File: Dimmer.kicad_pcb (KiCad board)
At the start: 2 copper layers, 129 x 68 mm, 62 parts, among them J1 220to12, J10 Detect_nullA, J11 220v_OUT, J12 Load_cntrlA, J13 ADC, J14 Conn_01x01, J15 Conn_01x01, J16 Conn_01x01, J17 Conn_01x01, J18 Conn_01x01, J19 Conn_01x01, J2 Prog, J22 SPI, J3 UART0, J4 Mode, J5 Load_cntrl, J6 Detect_null, J7 I2C, J8 ADC, J9 220v_IN, Q1 IRFP460APBF, Q2 IRFP460APBF, Q3 BC807, SW1 SW_Push, SW2 SW_Push, U2 ESP32-WROOM-32D, U3 L78L33_SO8, U4 TLP185, k1 Key, k2 Key, k3 Key, k4 Key, k5 Key, k6 Key, k7 Key

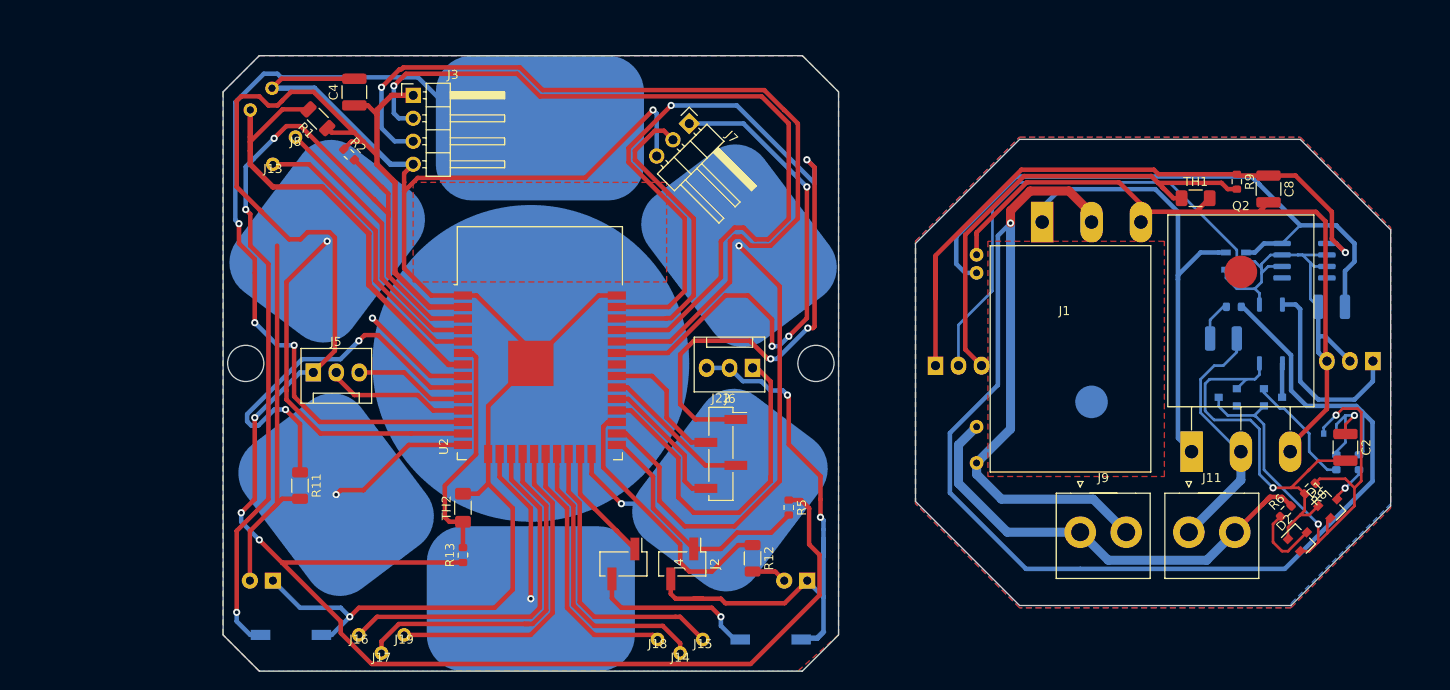
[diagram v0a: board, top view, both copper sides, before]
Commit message: Add files via upload
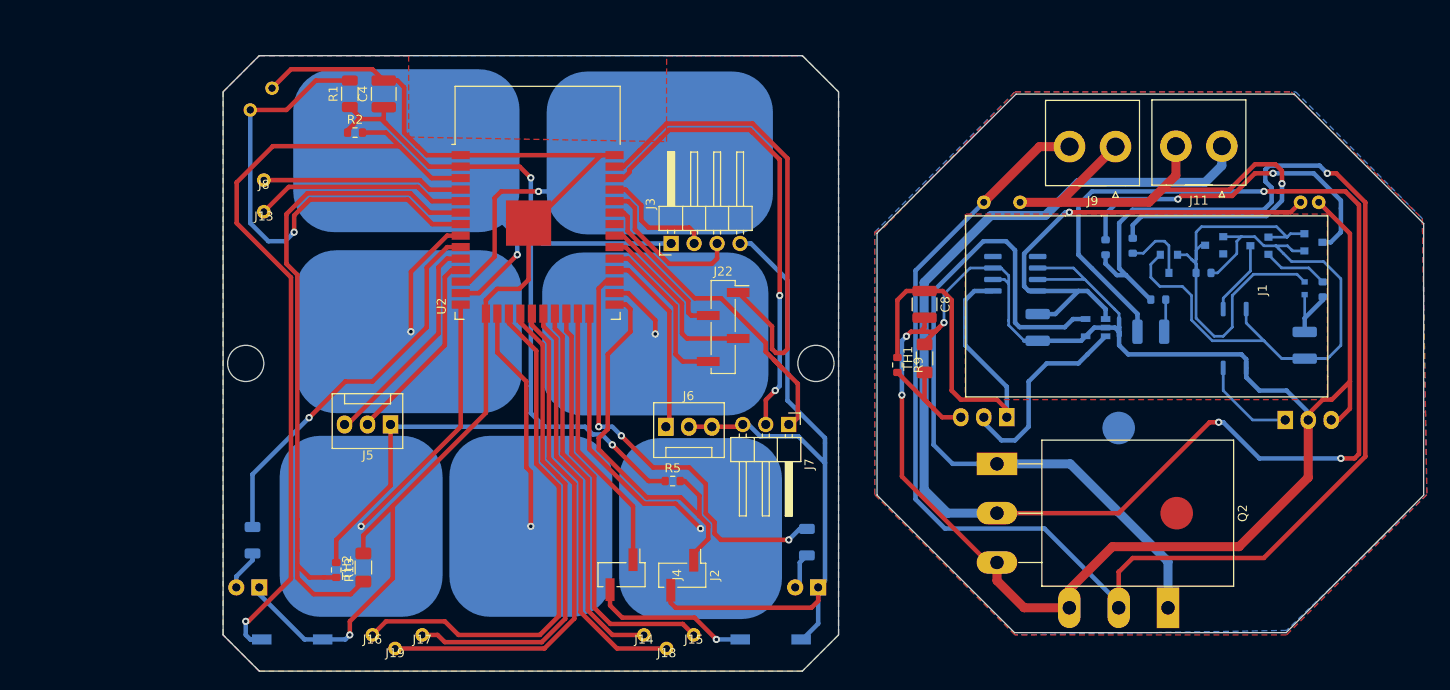
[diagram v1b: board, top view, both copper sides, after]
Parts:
- C2, D1, D2, R11, R12, R6, R8: moved to B.Cu
- moved Q1 44.8 mm to (207.4, 135.0), turned to 180 degrees
- moved R9 42.6 mm to (177.5, 108.2)
- moved C8 40.1 mm to (180.5, 101.5)
- moved J11 36.8 mm to (213.3, 87.0), turned to 180 degrees
- moved J9 36.8 mm to (201.6, 87.0), turned to 180 degrees
- moved R4 36.7 mm to (200.5, 95.2), turned to 270 degrees
- moved J7 35.0 mm to (165.5, 114.8), turned to 270 degrees
- moved TH1 34.8 mm to (180.5, 107.5), turned to 90 degrees
- moved R6 33.9 mm to (203.5, 95.0), turned to 90 degrees
- moved D2 33.7 mm to (207.5, 97.0), turned to 270 degrees
- moved J3 32.9 mm to (152.5, 94.8), turned to 90 degrees
- moved C11 32.6 mm to (193.0, 104.0), turned to 270 degrees
- moved U3 32.0 mm to (190.5, 98.1), turned to 0 degrees
- moved D1 29.2 mm to (223.5, 94.6), turned to 0 degrees
- moved R8 26.6 mm to (211.3, 98.0), turned to 0 degrees
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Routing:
- net Net-(C1-Pad2): track 28.0 -> 195.4 mm, vias 0 -> 3
- net +3V3: track 302.9 -> 172.6 mm, vias 4 -> 2
- net Net-(J3-Pad3): track 97.7 -> 17.5 mm, vias 1 -> 0
- net Net-(J3-Pad2): track 89.9 -> 12.9 mm, vias 1 -> 0
- net Net-(U2-Pad12): track 101.4 -> 31.7 mm, vias 3 -> 1
- net GND: track 362.0 -> 424.8 mm
- net Net-(U2-Pad26): track 58.4 -> 7.26 mm
- net MOSI: track 104.5 -> 53.6 mm, vias 4 -> 0
- net Net-(R13-Pad2): track 25.8 -> 75.3 mm
- net Net-(J12-Pad3): track 52.1 -> 12.8 mm
- net Net-(D5-Pad2): track 41.7 -> 4.49 mm
- net Net-(U2-Pad8): track 47.8 -> 13.8 mm
- net Net-(D1-Pad3): track 4.26 -> 38.0 mm, vias 1 -> 2
- net cntrl: track 53.2 -> 22.6 mm
- net Net-(D7-Pad5): track 52.5 -> 81.4 mm
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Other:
- board size 129 x 68 mm -> 132.7 x 68 mm

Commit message: Add files via upload
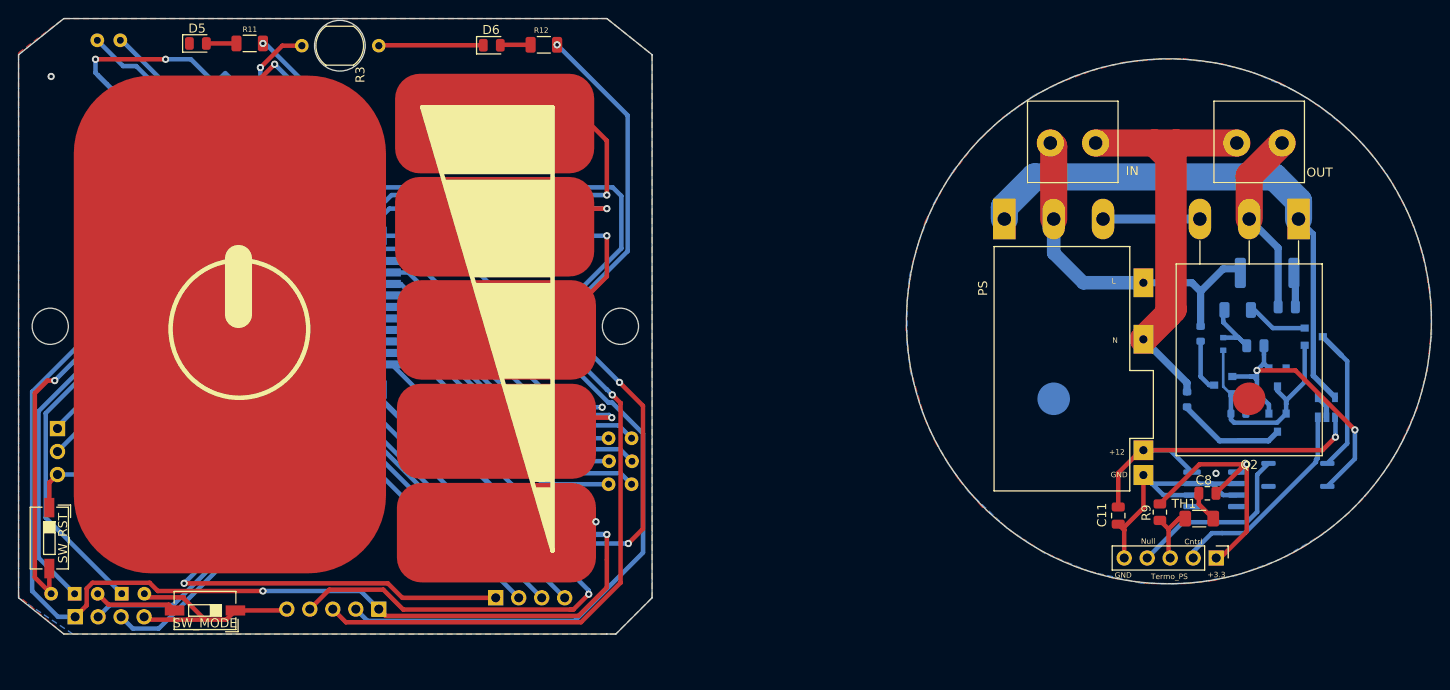
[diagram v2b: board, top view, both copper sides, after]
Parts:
- removed J1: 220to12, Touch_pad:oblast_bp
- removed J11: 220v_OUT, Touch_pad:220V_1x02_P5.08mm_Horizontal
- removed J17, J18, J19: Conn_01x01, Touch_pad:polz_razjem
- removed J2: Prog, Connector_PinHeader_2.54mm:PinHeader_1x02_P2.54mm_Vertical_SMD_Pin1Left
- removed J22: SPI, Connector_PinHeader_2.54mm:PinHeader_1x04_P2.54mm_Vertical_SMD_Pin1Right
- removed J7: I2C, Connector_PinHeader_2.54mm:PinHeader_1x03_P2.54mm_Horizontal
- removed J9: 220v_IN, Touch_pad:220V_1x02_P5.08mm_Horizontal
- removed k1: Key, Touch_pad:TestPoint_Pad_1.0x1.0sm
- added I2C: I2C, Connector_PinHeader_2.54mm:PinHeader_1x03_P2.54mm_Horizontal, B.Cu at (84.7, 115.2)
- added IN: 220v_IN, SMout:OUT_IN(1), F.Cu at (201.9, 78.9)
- added Mode: Mode, SMout:2pins, F.Cu at (89.1, 133.5)
- added OUT: 220v_OUT, SMout:OUT_IN(1), F.Cu at (222.5, 78.9)
- added PS: 220to12, SMout:oblast_bp, F.Cu at (188.2, 95.1)
- added Prog: , SMout:2pins, F.Cu at (89.8, 133.4)
- added RST: Reset, SMout:polz_razjem, F.Cu at (84.0, 133.4)
- added SPI: SPI, Connector_PinHeader_2.54mm:PinHeader_1x04_P2.54mm_Vertical, B.Cu at (133.1, 133.9)
- C1, C2, C8: footprint Capacitor_SMD:C_1210_3225Metric -> Capacitor_SMD:C_0805_2012Metric
- C11: footprint Capacitor_SMD:C_1210_3225Metric -> Capacitor_SMD:C_0805_2012Metric; moved to F.Cu
- C4, R1, R5, TH2, U2: moved to B.Cu
- D5, D6: footprint LED_THT:LED_D3.0mm_Clear -> LED_SMD:LED_0805_2012Metric; moved to F.Cu
- J10: value Detect_nullA -> Pin; footprint Connector:FanPinHeader_1x03_P2.54mm_Vertical -> SMout:polz_razjem; moved to F.Cu
- J12: value Load_cntrlA -> Pin; footprint Connector:FanPinHeader_1x03_P2.54mm_Vertical -> SMout:polz_razjem; moved to F.Cu
- J13, J8: footprint Touch_pad:polz_razjem -> SMout:polz_razjem; moved to B.Cu
- J14: value Conn_01x01 -> Pin; footprint Touch_pad:polz_razjem -> SMout:polz_razjem; moved to B.Cu
- J15: value Conn_01x01 -> Pin; footprint Touch_pad:polz_razjem -> SMout:polz_razjem
- J16: value Conn_01x01 -> Conn_01x05; footprint Touch_pad:polz_razjem -> Connector_PinHeader_2.54mm:PinHeader_1x05_P2.54mm_Vertical; moved to B.Cu
- J4: value Mode -> Conn_01x05; footprint Connector_PinHeader_2.54mm:PinHeader_1x02_P2.54mm_Vertical_SMD_Pin1Left -> Connector_PinHeader_2.54mm:PinHeader_1x05_P2.54mm_Vertical
- J5: value Load_cntrl -> Pin; footprint Connector:FanPinHeader_1x03_P2.54mm_Vertical -> SMout:polz_razjem
- J6: value Detect_null -> Pin; footprint Connector:FanPinHeader_1x03_P2.54mm_Vertical -> SMout:polz_razjem
- R10: footprint Resistor_SMD:R_0603_1608Metric -> Resistor_SMD:R_1206_3216Metric
- R11, R12, k2, k3, k4, k5, k6, k7: moved to F.Cu
- R13, R2: footprint Resistor_SMD:R_0603_1608Metric -> Resistor_SMD:R_0805_2012Metric; moved to B.Cu
- R3: footprint OptoDevice:R_LDR_5.1x4.3mm_P3.4mm_Vertical -> SMout:R_LDR_5.1x4.3mm_P3.4mm_Vertical; moved to F.Cu
- R7: footprint Resistor_SMD:R_0603_1608Metric -> Resistor_SMD:R_2512_6332Metric
- R9: footprint Resistor_SMD:R_0603_1608Metric -> Resistor_SMD:R_0805_2012Metric
- RX0: renamed from J3; footprint Connector_PinHeader_2.54mm:PinHeader_1x04_P2.54mm_Horizontal -> Connector_PinHeader_2.54mm:PinHeader_1x04_P2.54mm_Vertical; moved to B.Cu
- SW_MODE: renamed from SW2; moved to F.Cu
- SW_RST: renamed from SW1; moved to F.Cu
- moved RX0 77.7 mm to (86.7, 136.0), turned to 270 degrees
- moved J10 74.8 mm to (145.6, 116.3)
- moved D6 69.9 mm to (132.7, 72.8), turned to 0 degrees
- moved J4 65.7 mm to (212.7, 129.5)
- moved SW_MODE 62.6 mm to (101.0, 135.3)
- moved R12 62.2 mm to (138.4, 72.8), turned to 180 degrees
- moved D5 60.5 mm to (100.2, 72.7), turned to 0 degrees
- moved TH2 55.2 mm to (102.3, 77.7), turned to 45 degrees
- moved R11 54.9 mm to (105.9, 72.7), turned to 180 degrees
- moved R13 50.6 mm to (105.0, 81.3), turned to 225 degrees
- moved Q1 46.6 mm to (189.3, 92.0), turned to 0 degrees
- moved J12 44.2 mm to (145.6, 118.8), turned to 0 degrees
- moved Q2 42.9 mm to (221.8, 92.0), turned to 180 degrees
- moved C8 37.6 mm to (211.8, 122.3), turned to 180 degrees
- moved TH1 35.1 mm to (210.8, 125.2), turned to 0 degrees
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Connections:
- net GPIO35 renamed photo
- D7 pad 3: cntrl -> Load_cntrl
- J12 pad 1: +3V3 -> Net-(J12-Pad1)
- J16 pad 1: Net-(J16-Pad1) -> +3V3
- J4 pad 1: Mode -> +3V3
- J4 pad 2: Net-(J4-Pad2) -> Load_cntrl
- J5 pad 1: +3V3 -> Net-(J5-Pad1)
- J6 pad 1: GPIO17 -> Net-(J6-Pad1)
- R9 pad 2: Net-(J12-Pad3) -> Net-(J4-Pad3)
- SW_MODE pad 2: Net-(J4-Pad2) -> Net-(J23-Pad2)
- TH1 pad 1: Net-(J12-Pad3) -> Net-(J4-Pad3)
- U2 pad 10: GPIO32 -> termo_bp
- U2 pad 11: GPIO26 -> cntrl
- U2 pad 17: Net-(J16-Pad1) -> Net-(J6-Pad1)
- U2 pad 18: Net-(J17-Pad1) -> Net-(J10-Pad1)
- U2 pad 19: Net-(J19-Pad1) -> Net-(J15-Pad1)
- U2 pad 20: Net-(J18-Pad1) -> Net-(J12-Pad1)
- U2 pad 22: Net-(J15-Pad1) -> Net-(J5-Pad1)
- U2 pad 28: GPIO17 -> null
- U4 pad 6: Net-(J10-Pad1) -> Detect_null
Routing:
- net GND: track 424.8 -> 161.7 mm, vias 4 -> 3
- net Net-(C1-Pad2): track 195.4 -> 20.7 mm, vias 3 -> 0
- net Net-(J1-Pad1): track 188.5 -> 39.7 mm, vias 1 -> 0
- net termo_bp: track 0.00 -> 122.1 mm, vias 0 -> 1
- net +3V3: track 172.6 -> 258.1 mm, vias 2 -> 5
- net null: track 0.00 -> 70.9 mm, vias 0 -> 1
- net cntrl: track 22.6 -> 90.8 mm
- net Net-(J16-Pad1): track 58.4 -> 0.00 mm
- net Net-(J19-Pad1): track 56.8 -> 0.00 mm
- net Net-(R13-Pad2): track 75.3 -> 18.9 mm
- net Net-(J17-Pad1): track 53.0 -> 0.00 mm
- net RED: track 48.7 -> 101.4 mm
- net Net-(J18-Pad1): track 45.8 -> 0.00 mm
- net Net-(U2-Pad8): track 13.8 -> 51.6 mm
- net Net-(C2-Pad2): track 70.7 -> 35.9 mm, vias 0 -> 2
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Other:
- board size 132.7 x 68 mm -> 156.1 x 68 mm
- board text added: "+12"
- board text added: "+3.3"
- board text added: "CLK"
- board text added: "CS"
- board text added: "Cntrl"
- board text added: "GND"
- board text added: "L"
- board text added: "MISO"
- board text added: "MOSI"
- board text added: "N"
- board text added: "Null"
- board text added: "SCL"
- board text added: "SDA"
- board text added: "Sw_M"
- board text added: "TX0"
- board text added: "Termo_PS"
